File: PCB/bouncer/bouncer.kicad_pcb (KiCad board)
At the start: 2 copper layers, 15 parts, among them J1 Conn_01x08_Female, SW1 SW_Push_Dual, SW2 SW_Push_Dual, SW3 SW_Push_Dual, U1 74HC14

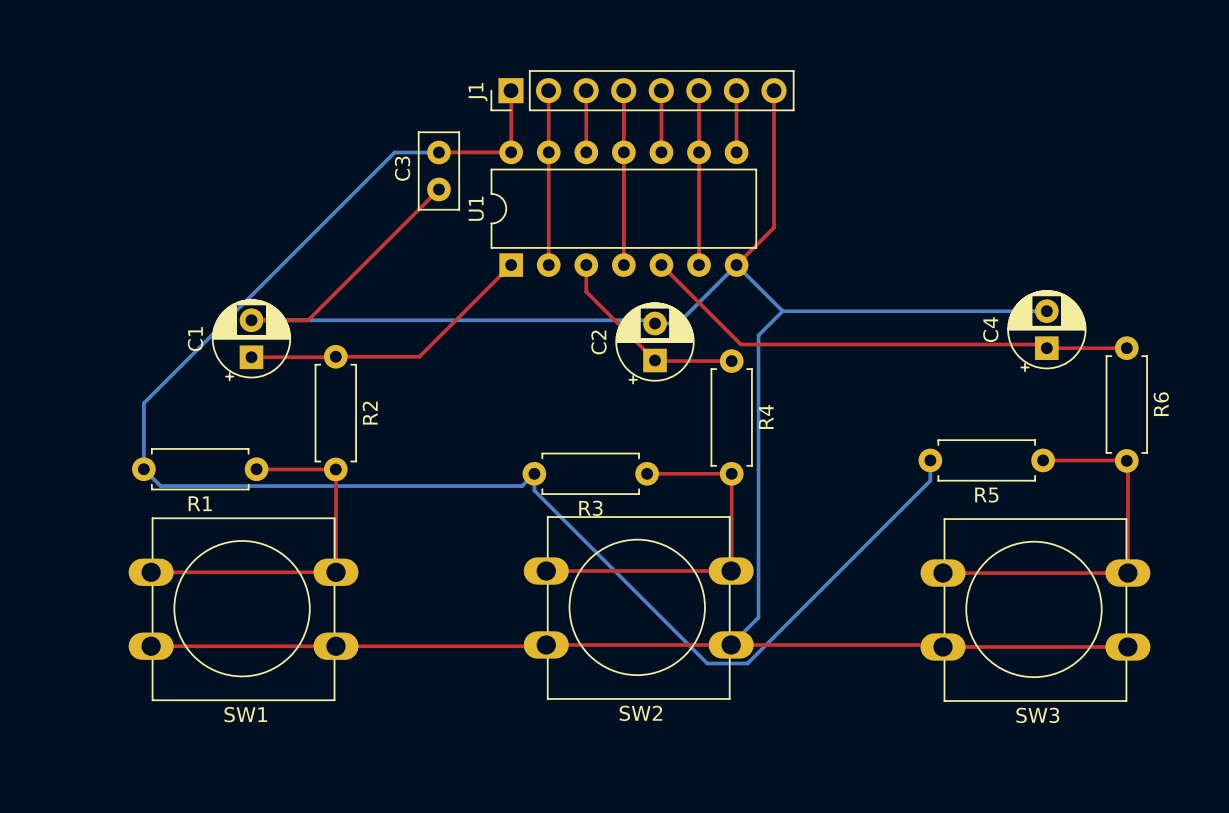
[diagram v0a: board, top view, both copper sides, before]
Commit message: Final changes for v2
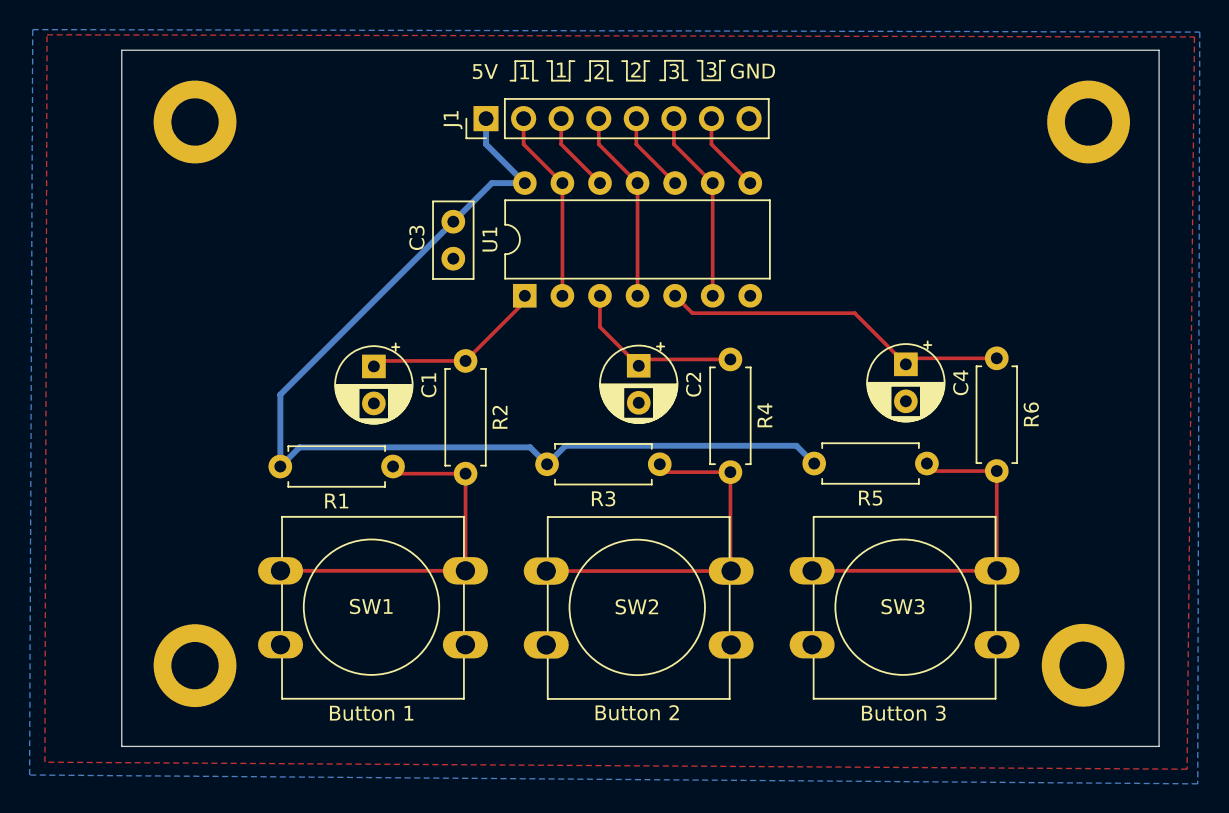
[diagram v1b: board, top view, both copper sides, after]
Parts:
- added ?: MountingHole_3.2mm_M3_DIN965_Pad, MountingHole:MountingHole_3.2mm_M3_DIN965_Pad, F.Cu at (189.6, 118.5)
- added ?: MountingHole_3.2mm_M3_DIN965_Pad, MountingHole:MountingHole_3.2mm_M3_DIN965_Pad, F.Cu at (129.6, 118.5)
- added ?: MountingHole_3.2mm_M3_DIN965_Pad, MountingHole:MountingHole_3.2mm_M3_DIN965_Pad, F.Cu at (190.0, 81.8)
- added ?: MountingHole_3.2mm_M3_DIN965_Pad, MountingHole:MountingHole_3.2mm_M3_DIN965_Pad, F.Cu at (129.6, 81.8)
- moved C4 9.59 mm to (177.6, 98.1), turned to -90 degrees
- moved R1 9.23 mm to (143.0, 105.1)
- moved SW3 8.85 mm to (183.8, 117.1)
- moved R6 8.82 mm to (183.8, 97.7)
- moved R2 8.78 mm to (147.9, 97.9)
- moved SW1 8.75 mm to (147.9, 117.1)
- moved C1 8.30 mm to (141.7, 98.3), turned to -90 degrees
- moved R5 7.86 mm to (179.1, 104.9)
- moved C3 4.78 mm to (147.1, 88.5)
- moved J1 2.53 mm to (149.3, 81.5)
- moved U1 2.27 mm to (151.9, 93.5)
- moved C2 1.16 mm to (159.6, 98.2), turned to -90 degrees
- moved R3 1.07 mm to (161.0, 104.9)
- moved R4 0.14 mm to (165.8, 97.8)
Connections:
- net ~BUTTON_1 renamed ~{BUTTON_1}
- net ~BUTTON_2 renamed ~{BUTTON_2}
- net ~BUTTON_3 renamed ~{BUTTON_3}
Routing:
- net GND: track 176.1 -> 0.00 mm
- net +5V: track 107.0 -> 70.9 mm
- net Net-(R6-Pad1): track 33.8 -> 23.8 mm
- net Net-(R2-Pad1): track 20.1 -> 12.4 mm
- net Net-(R5-Pad1): track 25.8 -> 24.2 mm
- net Net-(R4-Pad1): track 13.6 -> 12.2 mm
- net ~{BUTTON_3}: track 4.17 -> 5.44 mm
- net ~{BUTTON_2}: track 4.17 -> 5.44 mm
- net BUTTON_2: track 11.8 -> 13.1 mm
- net ~{BUTTON_1}: track 4.17 -> 5.44 mm
- net BUTTON_3: track 11.8 -> 13.1 mm
- net BUTTON_1: track 11.8 -> 13.1 mm
- net Net-(R1-Pad1): track 24.8 -> 24.2 mm
- net Net-(R3-Pad1): track 24.8 -> 24.2 mm
- added copper zone on B.Cu, net GND
- added copper zone on F.Cu, net GND
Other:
- board outline added: 70.1 x 47.1 mm
- net class Default removed
- board text added: "1"
- board text added: "2"
- board text added: "3"
- board text added: "5V"
- board text added: "Button 1"
- board text added: "Button 2"
- board text added: "Button 3"
- board text added: "GND"
